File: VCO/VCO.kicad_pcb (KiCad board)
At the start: 2 copper layers, 51 parts, among them J1 EuroPower, J2 CV, J3 Triangle, J4 Square, J5 CV3, J6 Ramp, Q1 BC547, Q2 BC547, Q3 BC547, Q4 MMDT3904, Q5 BC547, U1 TL082, U2 TL082, U3 TL082

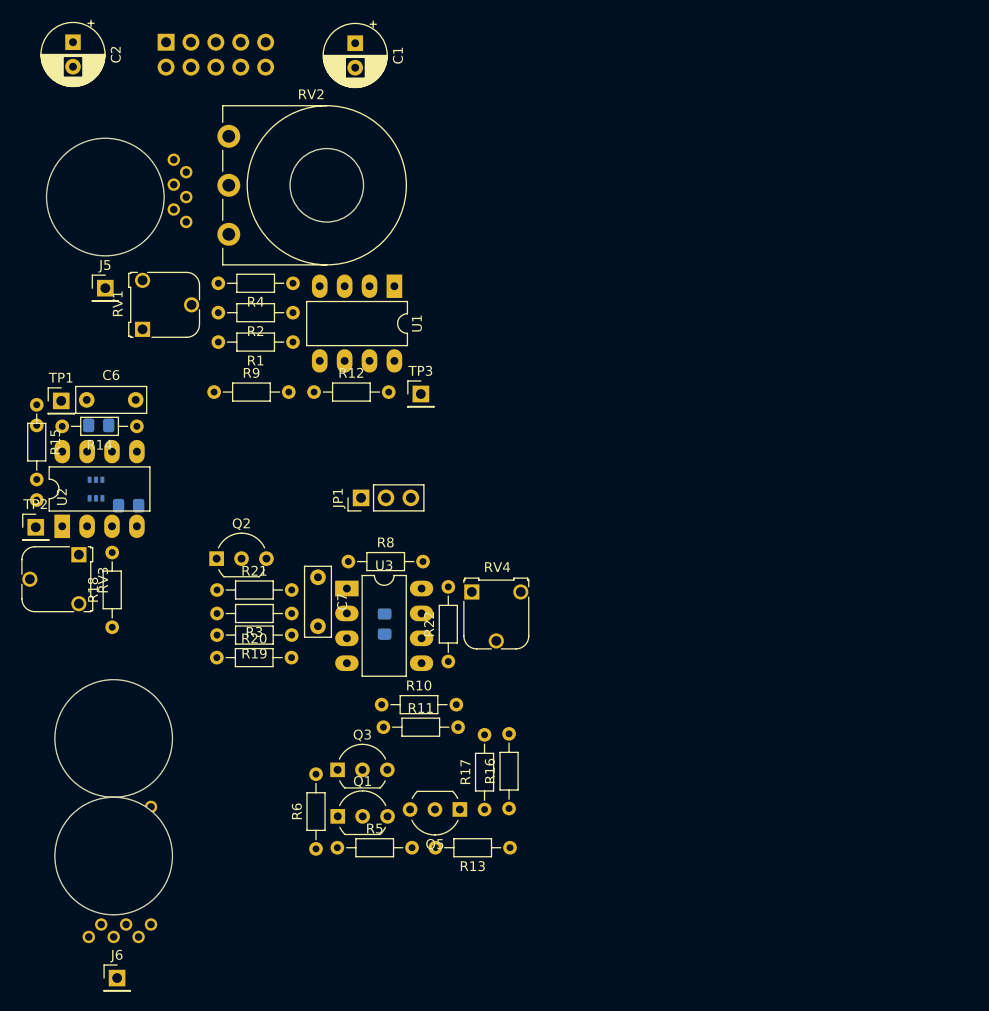
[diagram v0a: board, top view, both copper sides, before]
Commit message: VCO PCB
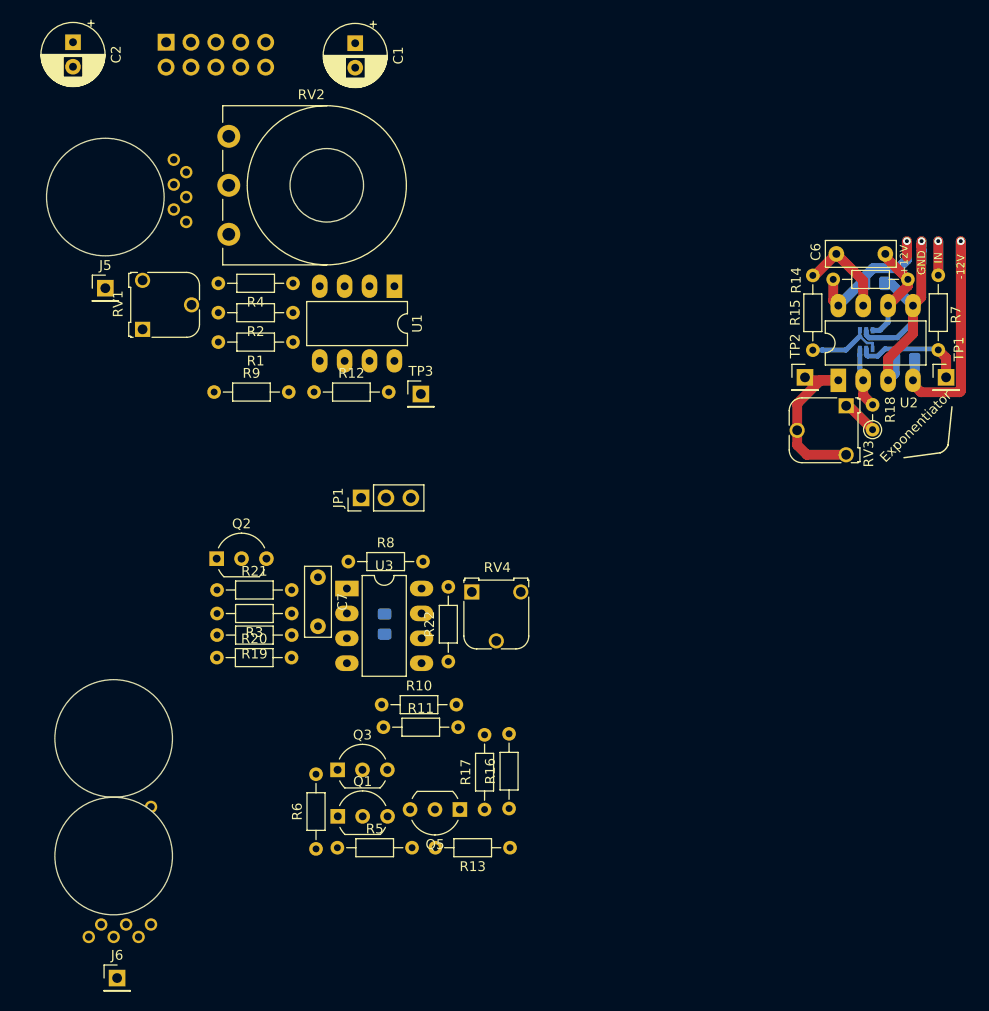
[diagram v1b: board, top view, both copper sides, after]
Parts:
- R18: footprint Resistor_THT:R_Axial_DIN0204_L3.6mm_D1.6mm_P7.62mm_Horizontal -> Resistor_THT:R_Axial_DIN0204_L3.6mm_D1.6mm_P2.54mm_Vertical
- R7: moved to F.Cu
- moved R7 93.3 mm to (103.8, 47.2)
- moved TP1 90.3 mm to (104.6, 50.0)
- moved C4 80.6 mm to (100.4, 48.2)
- moved U2 80.6 mm to (93.6, 50.3)
- moved C3 80.5 mm to (97.3, 40.4)
- moved R15 80.3 mm to (91.0, 39.6)
- moved R18 80.2 mm to (97.1, 55.3)
- moved R14 80.1 mm to (100.7, 40.0)
- moved Q4 80.1 mm to (96.5, 46.1)
- moved TP2 80.0 mm to (90.2, 50.0)
- moved RV3 79.8 mm to (94.4, 52.9)
- moved C6 77.9 mm to (93.4, 37.4)
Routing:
- net GND: track 0.00 -> 39.5 mm, vias 0 -> 1
- net -12V: track 0.00 -> 25.5 mm, vias 0 -> 1
- net /Vexp: track 0.00 -> 18.3 mm
- net +12V: track 0.00 -> 15.7 mm, vias 0 -> 1
- net Net-(C6-Pad2): track 0.00 -> 14.2 mm
- net Net-(Q4-Pad1): track 0.00 -> 13.6 mm
- net /CV: track 0.00 -> 12.1 mm
- net Net-(Q4-Pad3): track 0.00 -> 9.74 mm
- net Net-(C6-Pad1): track 0.00 -> 9.73 mm
- net Net-(R7-Pad2): track 0.00 -> 6.96 mm, vias 0 -> 1
- net Net-(R18-Pad1): track 0.00 -> 3.71 mm
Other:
- net class Default: clearance 0.2 -> 0.1524; trace_width 0.25 -> 0.1524; via_dia 0.8 -> 0.6858; via_drill 0.4 -> 0.3302
- rule trace_clearance: 0.2 -> 0.1524
- rule trace_min: 0.2 -> 0.1524
- rule via_min_drill: 0.3 -> 0.254
- rule via_min_size: 0.4 -> 0.508
- board text added: "+12V"
- board text added: "-12V"
- board text added: "Exponentiator"
- board text added: "GND"
- board text added: "IN"
